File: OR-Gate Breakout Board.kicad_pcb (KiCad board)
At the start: 2 copper layers, 5.5 x 5.4 mm, 8 parts, among them U5 74LVC1G332GW,125

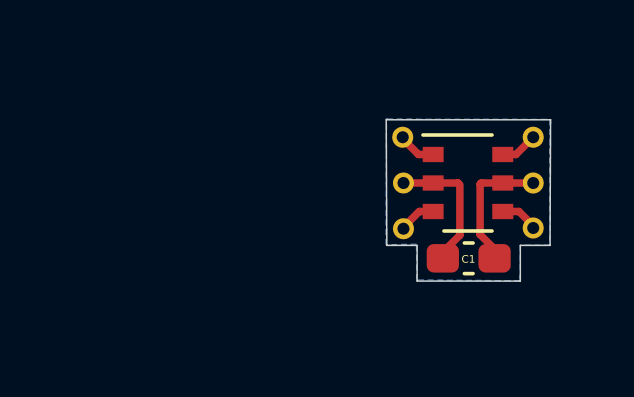
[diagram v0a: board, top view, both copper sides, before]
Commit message: Updated design to be a little more usable. Still need to consider resistors and stuff. Do not use this version. WIP
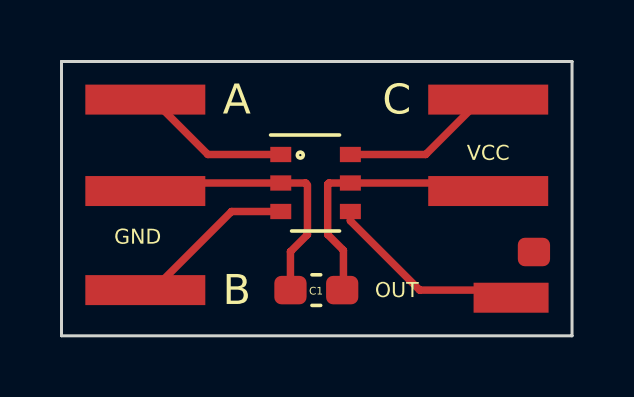
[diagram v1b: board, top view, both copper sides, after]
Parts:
- added ?: , , F.Cu at (155.2, 97.8)
- moved ? 8.84 mm to (142.2, 99.1)
- moved ? 8.67 mm to (142.2, 92.7)
- moved ? 8.61 mm to (142.2, 95.8)
- moved C1 5.19 mm to (147.9, 99.1)
- moved U5 5.08 mm to (147.9, 95.5)
- moved ? 2.44 mm to (154.4, 99.3)
- moved ? 1.96 mm to (153.7, 92.7)
- moved ? 1.52 mm to (153.7, 95.8)
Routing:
- net GND: track 4.08 -> 8.85 mm
- net VCC: track 4.46 -> 8.88 mm
- net OUT: track 1.25 -> 5.61 mm
- net B: track 1.17 -> 5.35 mm
- net C: track 1.25 -> 5.10 mm
- net A: track 1.23 -> 5.02 mm
- removed copper zone on B.Cu, net GND
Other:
- board size 5.5 x 5.4 mm -> 17 x 9.1 mm
- board text added: "A"
- board text added: "B"
- board text added: "C"
- board text added: "GND"
- board text added: "OUT"
- board text added: "VCC"
